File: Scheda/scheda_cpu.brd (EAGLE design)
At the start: 66.1 x 70 mm, 38 parts, among them IC2 LM3801N, IC3 LD1117V33

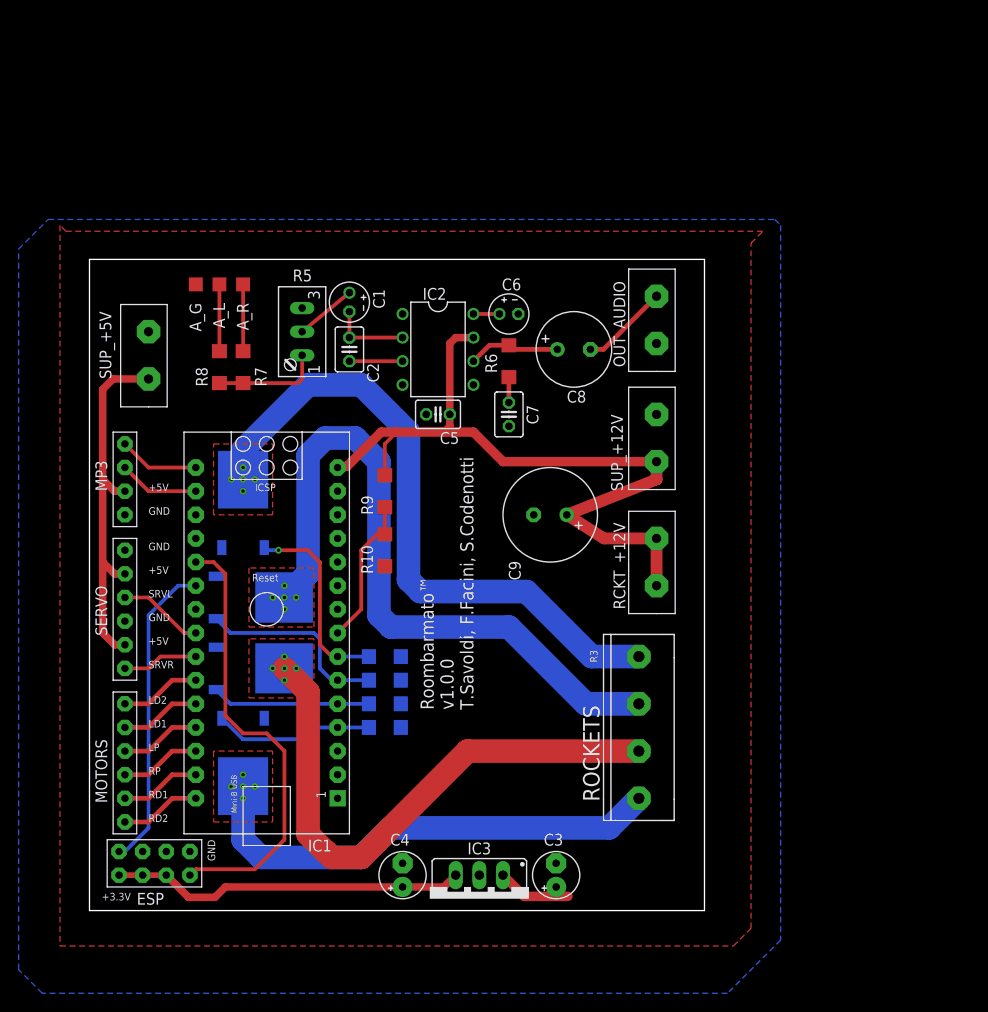
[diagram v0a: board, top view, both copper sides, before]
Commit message: modificato pcb
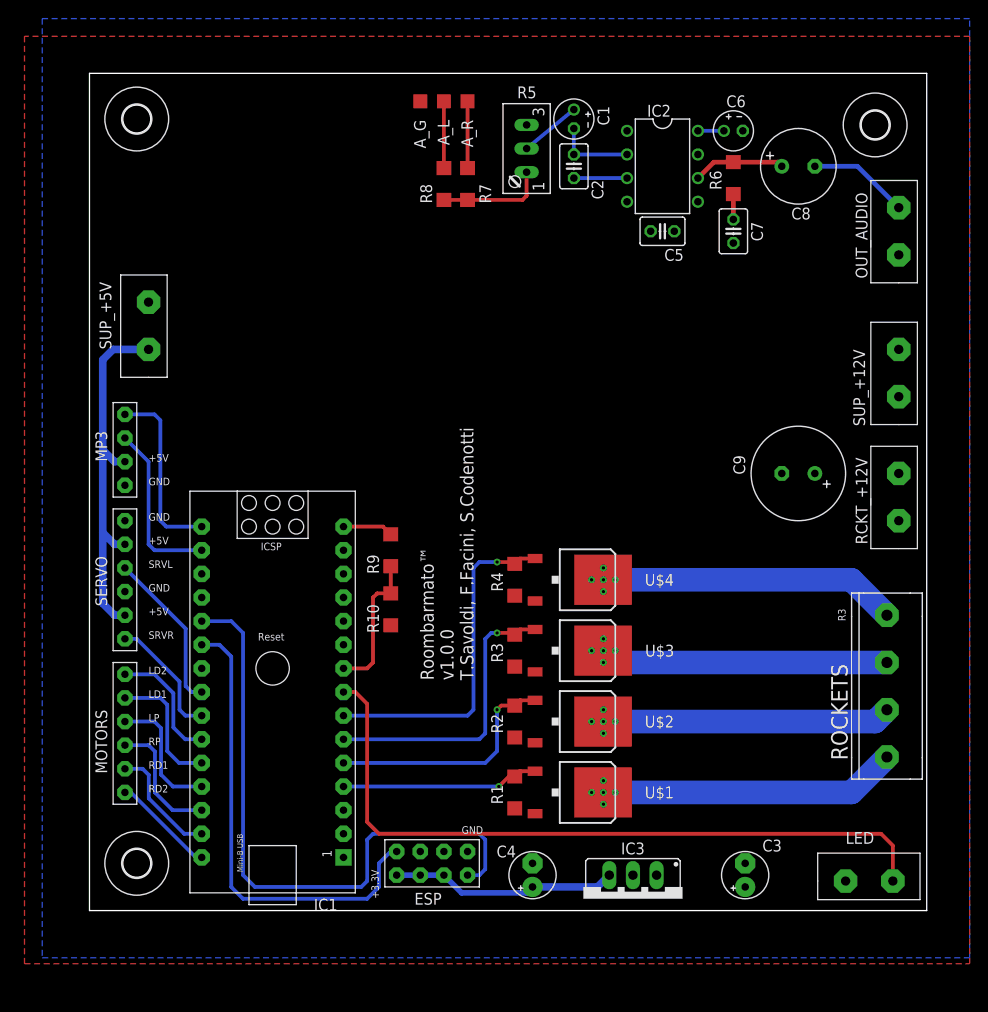
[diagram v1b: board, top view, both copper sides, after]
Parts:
- added H1, H2, H3: MOUNT-HOLE3.0, ITIS:3,0
- added LED: AK500, roombarmato_eagle_lib:AK500-2
- moved U$4 37.1 mm to (52.7, 35.6), flipped to the top, turned to 270 degrees
- moved U$1 36.3 mm to (52.7, 12.7), flipped to the top, turned to 270 degrees
- moved U$2 34.8 mm to (52.7, 20.3), flipped to the top, turned to 270 degrees
- moved U$3 34.8 mm to (52.7, 27.9), flipped to the top, turned to 270 degrees
- moved R5 31.1 mm to (45.7, 81.9)
- moved A_G 31.1 mm to (35.6, 87.0)
- moved A_L 31.1 mm to (38.1, 87.0)
- moved C7 31.1 mm to (69.2, 73.0)
- moved C8 31.1 mm to (76.2, 80.0)
- moved R8 31.1 mm to (38.1, 78.1)
- moved A_R 31.1 mm to (40.6, 87.0)
- moved C1 31.1 mm to (52.1, 85.1)
- moved C2 31.1 mm to (52.1, 80.0)
- moved R6 31.1 mm to (69.2, 78.7)
- moved R7 31.1 mm to (40.6, 78.1)
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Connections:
- net CHK_VBAT: now also IC1.9; no longer IC1.8
- net GND: now also LED.P$1
- net LED: now also IC1.8, LED.P$2; no longer IC1.9
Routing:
- net +12V: track 94.0 -> 5.42 mm
- net LED: track 0.00 -> 77.1 mm
- net R3: track 70.1 -> 35.9 mm
- net R2: track 74.2 -> 41.2 mm
- net R1: track 60.2 -> 40.0 mm
- net N$4: track 48.1 -> 68.1 mm
- net N$1: track 33.5 -> 50.4 mm
- net C_R3: track 21.3 -> 36.7 mm
- net +3.3V: track 38.2 -> 24.4 mm
- net RXD: track 8.67 -> 19.6 mm
- net C_R2: track 21.0 -> 31.6 mm, vias 0 -> 1
- net TXD: track 8.67 -> 18.5 mm
- net R0: track 51.7 -> 42.4 mm
- net C_R1: track 17.1 -> 26.0 mm, vias 0 -> 1
- net SRV_L: track 9.20 -> 17.4 mm
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- added copper zone on layer 16, net +12V
- added copper zone on layer 1, net GND
- removed copper zone on layer 1, net +12V
- removed copper zone on layer 16, net GND
- removed copper zone on layer 1, net R0
- removed copper zone on layer 1, net R1
- removed copper zone on layer 1, net R2
- removed copper zone on layer 1, net R3
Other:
- board size 66.1 x 70 mm -> 90 x 90 mm
